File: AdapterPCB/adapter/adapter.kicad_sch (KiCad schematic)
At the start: 5 parts, among them U1 SN74LVC245APW, U2 SN74LVC245APW

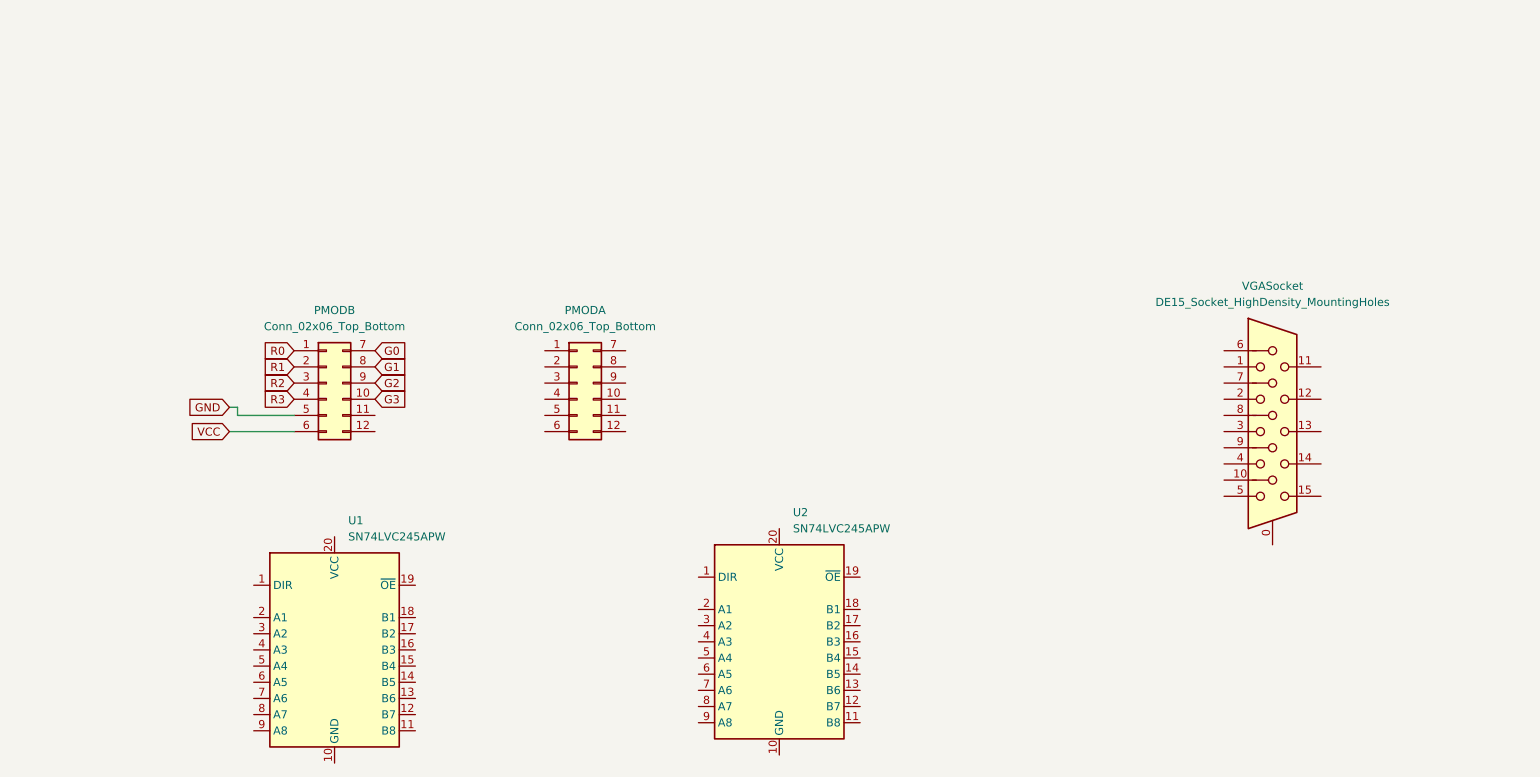
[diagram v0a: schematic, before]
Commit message: y
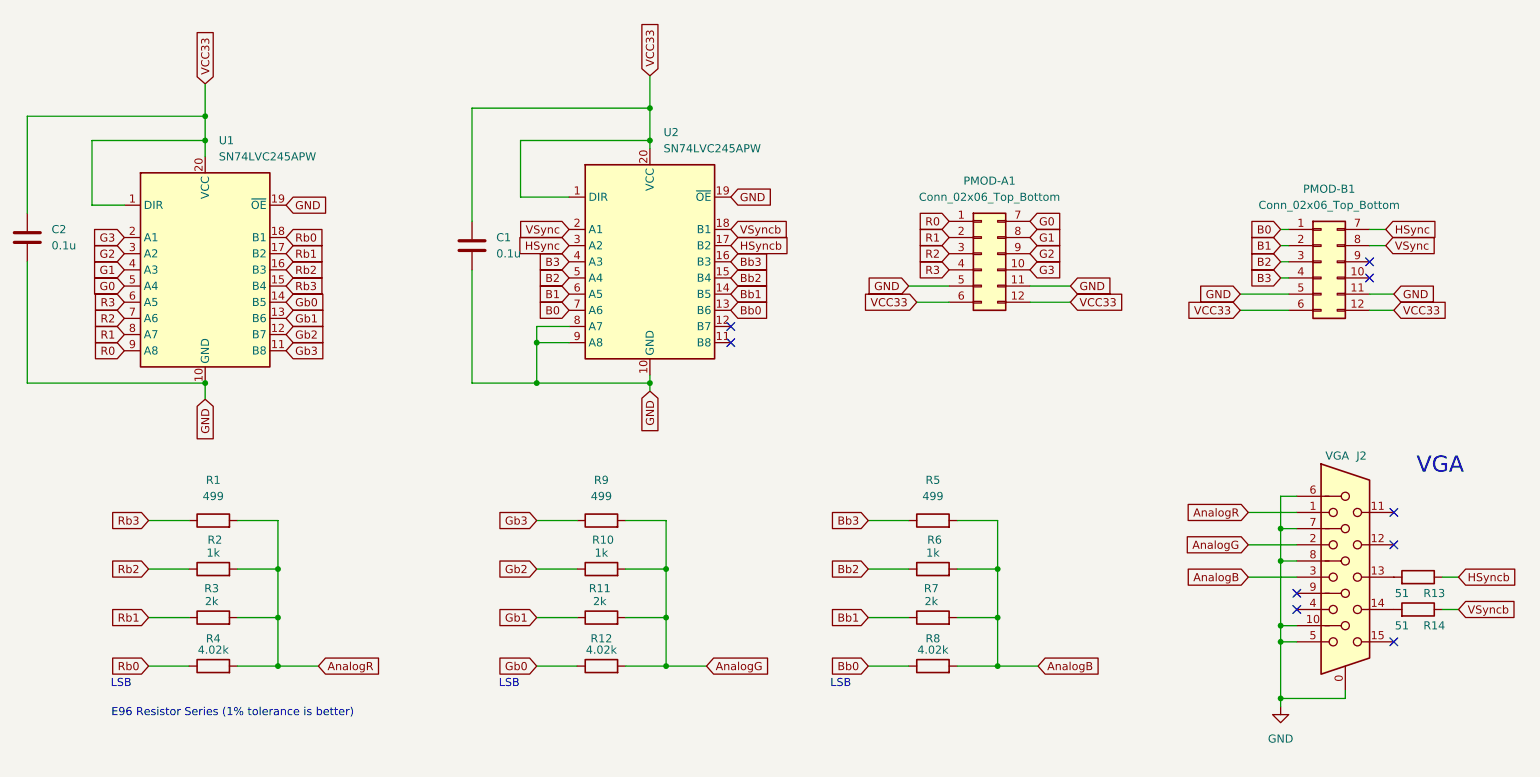
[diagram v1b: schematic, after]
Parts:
- removed VGASocket: DE15_Socket_HighDensity_MountingHoles, symbol Connector:DE15_Socket_HighDensity_MountingHoles
- added C1, C2: 0.1u, Capacitor_SMD:C_1808_4520Metric, symbol Device:C
- added J2: VGA, Connector_Dsub:DSUB-15-HD_Socket_Horizontal_P2.29x2.54mm_EdgePinOffset8.35mm_Housed_MountingHolesOffset10.89mm, symbol Connector:DE15_Receptacle_HighDensity_MountingHoles
- added R1, R5, R9: 499, Resistor_SMD:R_2010_5025Metric_Pad1.40x2.65mm_HandSolder, symbol Device:R
- added R10, R2, R6: 1k, Resistor_SMD:R_2010_5025Metric_Pad1.40x2.65mm_HandSolder, symbol Device:R
- added R11, R3, R7: 2k, Resistor_SMD:R_2010_5025Metric_Pad1.40x2.65mm_HandSolder, symbol Device:R
- added R12, R4, R8: 4.02k, Resistor_SMD:R_2010_5025Metric_Pad1.40x2.65mm_HandSolder, symbol Device:R
- added R13, R14: 51, Resistor_SMD:R_2010_5025Metric_Pad1.40x2.65mm_HandSolder, symbol Device:R
- PMOD-A1: renamed from PMODB; footprint (none) -> Connector_PinHeader_2.54mm:PinHeader_2x06_P2.54mm_Horizontal
- PMOD-B1: renamed from PMODA; footprint (none) -> Connector_PinHeader_2.54mm:PinHeader_2x06_P2.54mm_Horizontal
- U1, U2: footprint Package_SO:TSSOP-20_4.4x6.5mm_P0.65mm -> Package_SO:SOIC-20W_7.5x12.8mm_P1.27mm
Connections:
- net VCC is gone; now on net VCC33: PMOD-A1.6 (Pin_6)
- net G0: now also U1.5 (A4)
- net G1: now also U1.4 (A3)
- net G2: now also U1.3 (A2)
- net G3: now also U1.2 (A1)
- net GND: now also PMOD-A1.11 (Pin_11), PMOD-B1.11 (Pin_11), PMOD-B1.5 (Pin_5), U1.10 (GND), U1.19 (~{OE}), U2.10 (GND), U2.19 (~{OE}), U2.8 (A7), U2.9 (A8), C1.2, C2.2, J2.0, J2.10, J2.5, J2.6, J2.7, J2.8
- net R0: now also U1.9 (A8)
- net R1: now also U1.8 (A7)
- net R2: now also U1.7 (A6)
- net R3: now also U1.6 (A5)
- net VCC33: now reaches PMOD-A1.12 (Pin_12)
- net VCC33: now also PMOD-B1.12 (Pin_12), PMOD-B1.6 (Pin_6), U1.1 (DIR), U1.20 (VCC), U2.1 (DIR), U2.20 (VCC), C1.1, C2.1
- net B0: now reaches PMOD-B1.1 (Pin_1)
- net B0: now also U2.7 (A6)
- net B1: now reaches PMOD-B1.2 (Pin_2)
- net B1: now also U2.6 (A5)
- net B2: now reaches PMOD-B1.3 (Pin_3)
- net B2: now also U2.5 (A4)
- net B3: now reaches PMOD-B1.4 (Pin_4)
- net B3: now also U2.4 (A3)
- net HSync: now reaches PMOD-B1.7 (Pin_7)
- net HSync: now also U2.3 (A2)
- net VSync: now reaches PMOD-B1.8 (Pin_8)
- net VSync: now also U2.2 (A1)
- net Bb0: now reaches U2.13 (B6)
- net Bb0: now also R8.1
- net Bb1: now reaches U2.14 (B5)
- net Bb1: now also R7.1
- net Bb2: now reaches U2.15 (B4)
- net Bb2: now also R6.1
- net Bb3: now reaches U2.16 (B3)
- net Bb3: now also R5.1
- net HSyncb: now reaches U2.17 (B2)
- net HSyncb: now also R13.1
- net VSyncb: now reaches U2.18 (B1)
- net VSyncb: now also R14.1
- net Gb3: now reaches U1.11 (B8)
- net Gb3: now also R9.1
- net Gb2: now reaches U1.12 (B7)
- net Gb2: now also R10.1
- net Gb1: now reaches U1.13 (B6)
- net Gb1: now also R11.1
- net Gb0: now reaches U1.14 (B5)
- net Gb0: now also R12.1
- net Rb3: now reaches U1.15 (B4)
- net Rb3: now also R1.1
- net Rb2: now reaches U1.16 (B3)
- net Rb2: now also R2.1
- net Rb1: now reaches U1.17 (B2)
- net Rb1: now also R3.1
- net Rb0: now reaches U1.18 (B1)
- net Rb0: now also R4.1
- new net: J2.14, R14.2
- new net: J2.13, R13.2
- new net AnalogB: J2.3, R5.2, R6.2, R7.2, R8.2
- new net AnalogG: J2.2, R10.2, R11.2, R12.2, R9.2
- new net AnalogR: J2.1, R1.2, R2.2, R3.2, R4.2
- no-connect marks 0 -> 9
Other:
- note added: "E96 Resistor Series (1% tolerance is better)"
- note added: "LSB"
- note added: "VGA"
- moved on the sheet: PMOD-A1, PMOD-B1, U1, U2
